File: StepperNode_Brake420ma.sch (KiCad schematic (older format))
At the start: 15 parts, among them P12 TE_640456-8, U21 RCV420JP, U22 RCV420JP

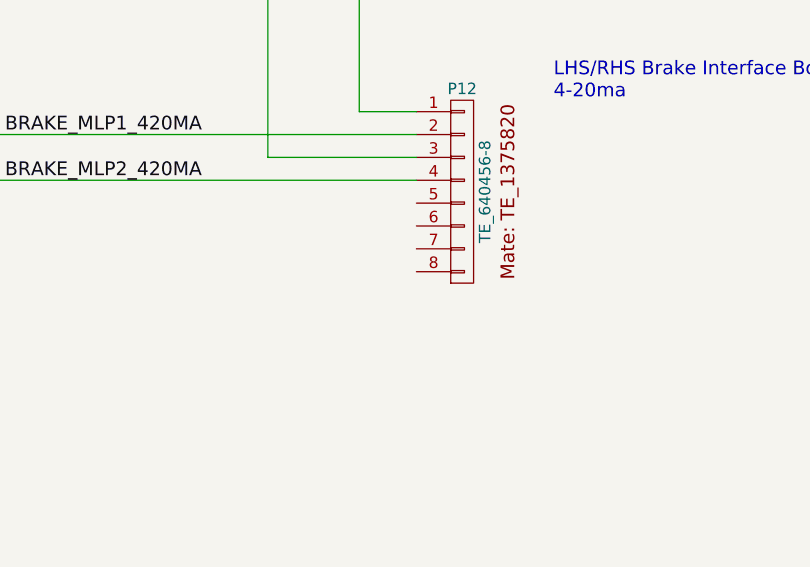
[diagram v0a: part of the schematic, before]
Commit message: Update per design review.
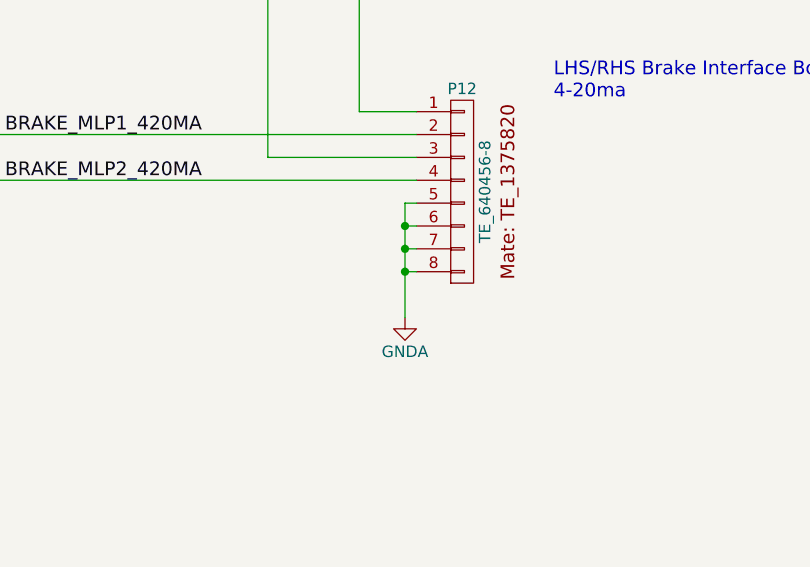
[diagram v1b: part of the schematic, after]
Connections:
- wire segments 25 -> 30
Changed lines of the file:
@@
 Wire Wire Line
 	10700 2600 11350 2600
+$Comp
+L GNDA #PWR?
+U 1 1 575D1FD8
+P 11300 3300
+F 0 "#PWR?" H 11300 3050 50  0001 C CNN
+F 1 "GNDA" H 11300 3150 50  0000 C CNN
+F 2 "" H 11300 3300 50  0000 C CNN
+F 3 "" H 11300 3300 50  0000 C CNN
+	1    11300 3300
+	1    0    0    -1
+$EndComp
+Wire Wire Line
+	11350 2800 11300 2800
+Wire Wire Line
+	11300 2800 11300 3300
+Wire Wire Line
+	11350 3100 11300 3100
+Connection ~ 11300 3100
+Wire Wire Line
+	11350 3000 11300 3000
+Connection ~ 11300 3000
+Wire Wire Line
+	11350 2900 11300 2900
+Connection ~ 11300 2900
 $EndSCHEMATC
